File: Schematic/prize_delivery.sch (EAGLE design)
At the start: 13 parts, among them Q1 IRL540

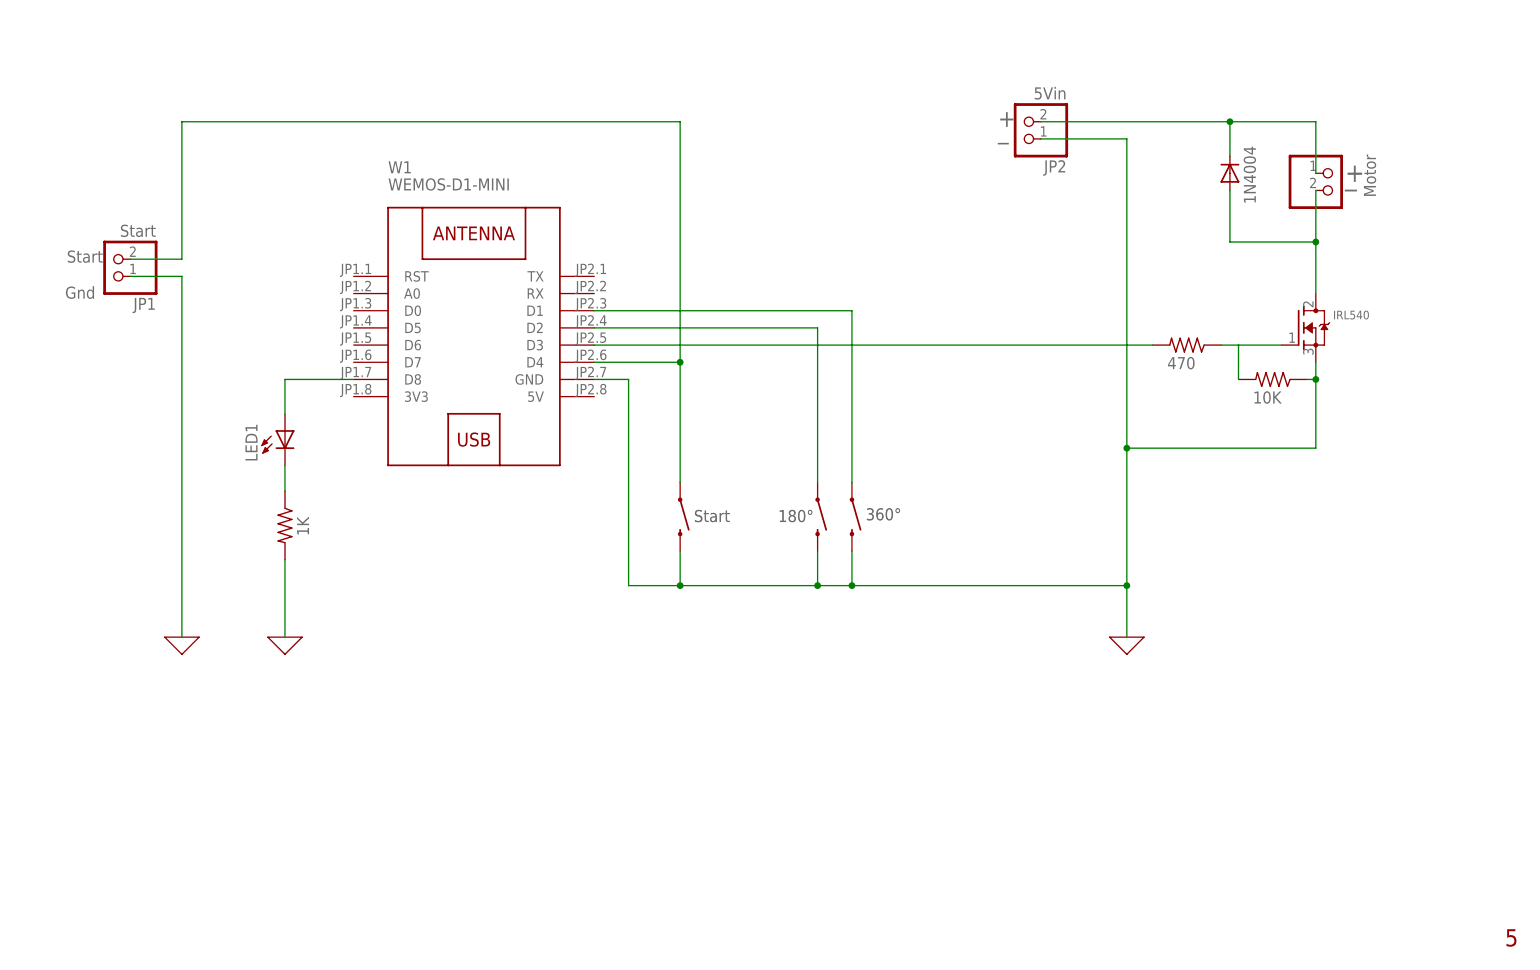
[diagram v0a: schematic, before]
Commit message: Modified schematic
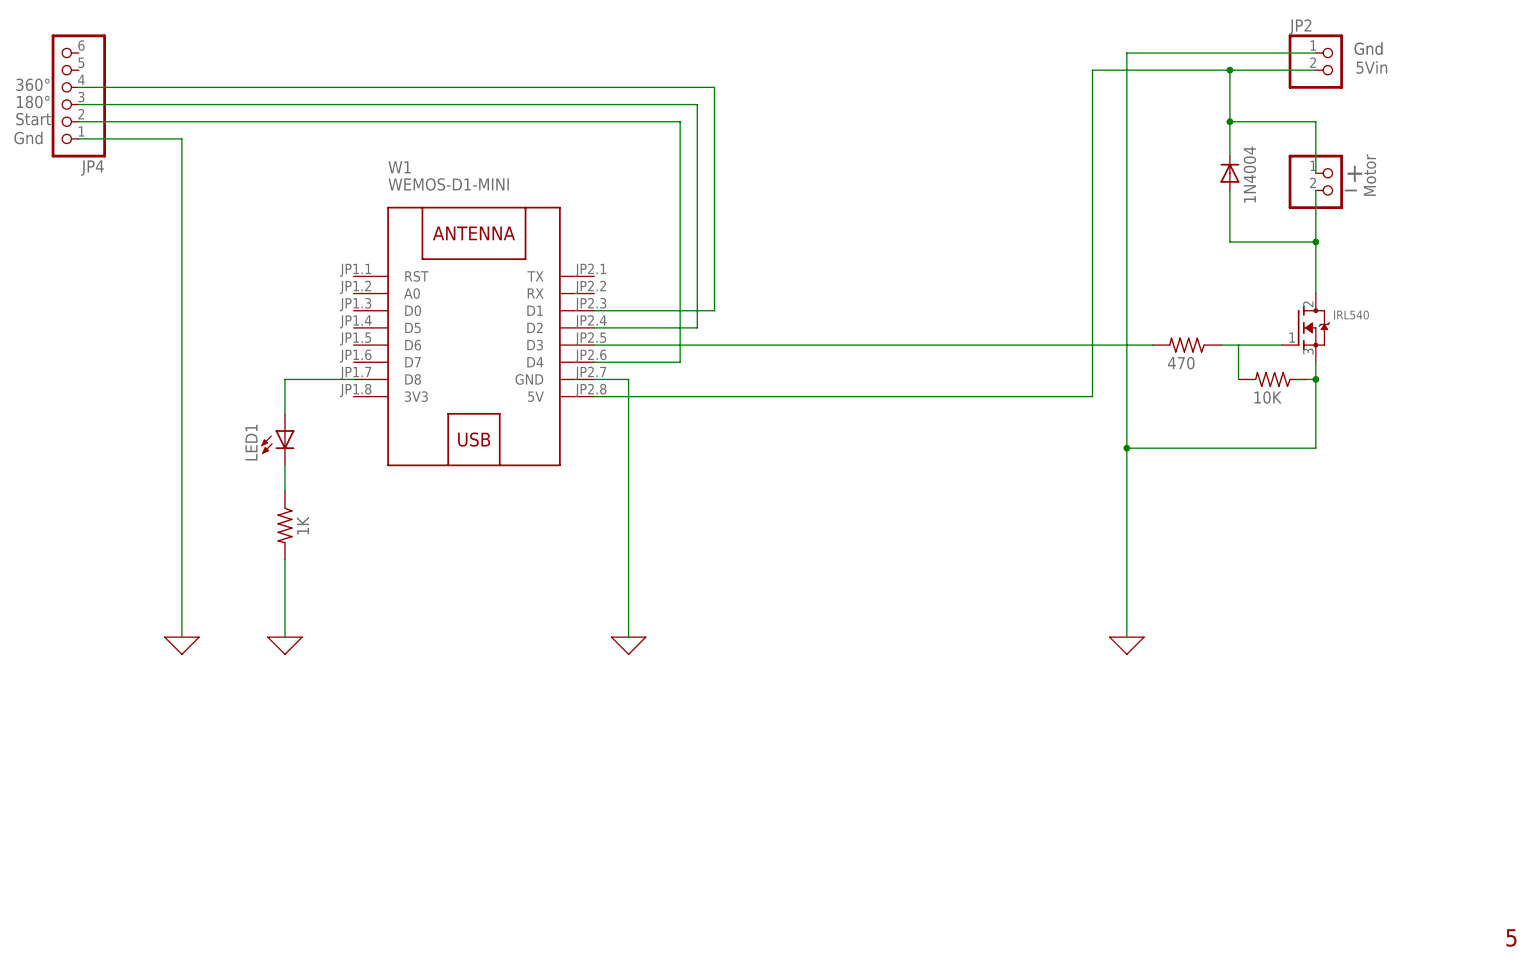
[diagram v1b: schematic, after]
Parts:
- removed 180°, 360°, START: MOMENTARY-SWITCH-SPST-PTH-6.0MM, SparkFun-Switches:MOMENTARY-SWITCH-SPST-PTH-6.0MM
- removed JP1: Start, pinhead:PINHD-1X2
- added JP4: (no value), adafruit:PINHD-1X6
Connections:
- net 0: now also JP4.1; no longer 180°.2, 360°.2, JP1.1, START.2
- net N$3: now also W1.5V
- net N$4: now also JP4.3; no longer 180°.1
- net N$5: now also JP4.4; no longer 360°.1
- net N$9: now also JP4.2; no longer JP1.2, START.1
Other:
- moved on the sheet: JP2

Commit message: Update PCB
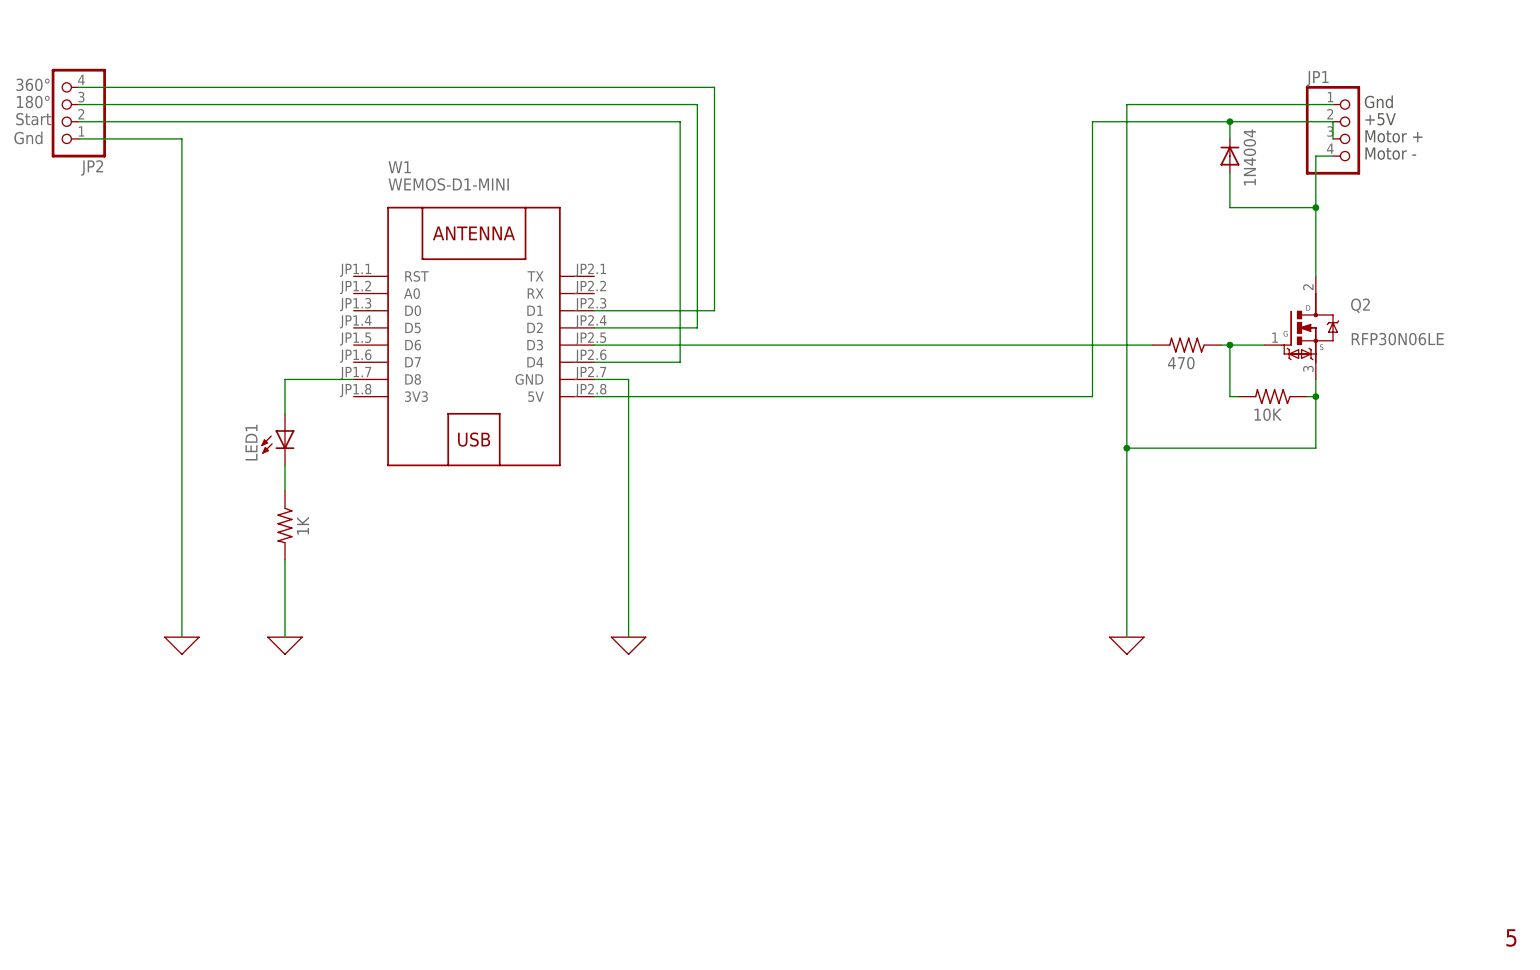
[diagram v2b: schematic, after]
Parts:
- removed JP3: Motor, pinhead:PINHD-1X2
- removed JP4: (no value), adafruit:PINHD-1X6
- removed Q1: IRL540, adafruit:MOSFET-NGDS_TO220V
- added JP1: (no value), pinhead:PINHD-1X4
- added Q2: RFP30N06LE, RFP30N06LE:RFP30N06LE
- JP2: value 5Vin -> (none); device pinhead:PINHD-1X2 -> pinhead:PINHD-1X4
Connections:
- removed net N$14: Q1.G, R2.1, R4.2
- new net N$8: Q2.G, R2.1, R4.2
- net 0: now also JP1.1, Q2.S; no longer JP4.1, Q1.S
- net N$2: now also JP1.4, Q2.D; no longer JP3.2, Q1.D
- net N$3: now also JP1.2, JP1.3; no longer JP2.2, JP3.1
- net N$4: now also JP2.3; no longer JP4.3
- net N$5: now also JP2.4; no longer JP4.4
- net N$9: now also JP2.2; no longer JP4.2
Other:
- note added: "+5V"
- note added: "Motor +"
- note added: "Motor -"
- note removed: "+"
- note removed: "_"
